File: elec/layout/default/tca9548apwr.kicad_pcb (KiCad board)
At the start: 2 copper layers, 20 parts

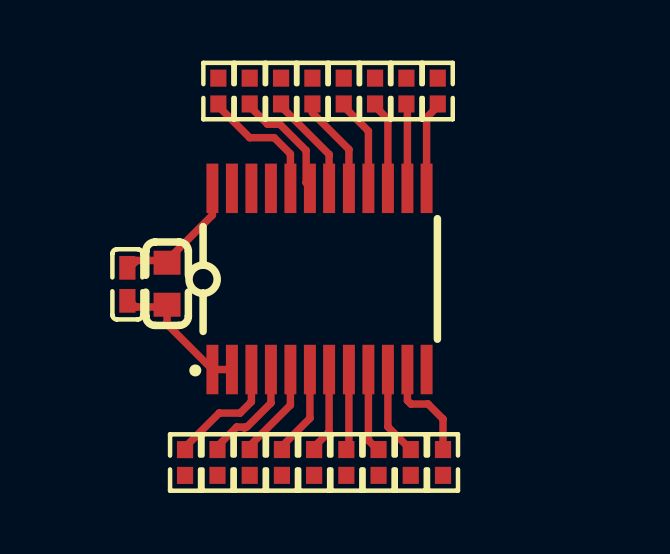
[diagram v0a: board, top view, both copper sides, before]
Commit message: Fix frozen
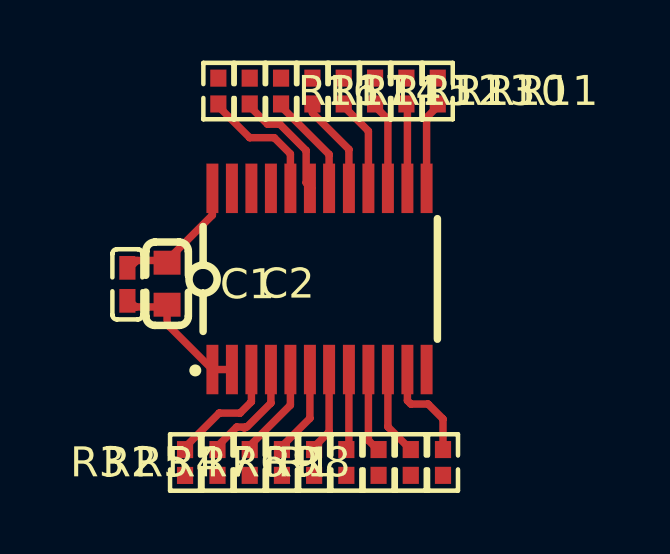
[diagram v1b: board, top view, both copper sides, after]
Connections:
- R1 pad 1: RESET_ -> line-13
- R10 pad 1: hv -> line-10
- R10 pad 2: line-1 -> hv
- R11 pad 1: hv -> line-8
- R11 pad 2: line-13 -> hv
- R12 pad 1: hv -> line
- R12 pad 2: line-5 -> hv
- R13 pad 1: hv -> line-16
- R13 pad 2: line-7 -> hv
- R14 pad 1: hv -> line-2
- R14 pad 2: line-14 -> hv
- R15 pad 1: hv -> line-3
- R15 pad 2: line-10 -> hv
- R16 pad 1: hv -> line-5
- R16 pad 2: line-9 -> hv
- R17 pad 1: hv -> line-15
- R17 pad 2: line-8 -> hv
- R2 pad 1: hv -> line-14
- R2 pad 2: line -> hv
- R3 pad 1: hv -> line-4
- R3 pad 2: line-15 -> hv
- R4 pad 1: hv -> line-12
- R4 pad 2: line-12 -> hv
- R5 pad 1: hv -> line-1
- R5 pad 2: line-4 -> hv
- R6 pad 1: hv -> line-9
- R6 pad 2: line-3 -> hv
- R7 pad 1: hv -> line-7
- R7 pad 2: line-11 -> hv
- R8 pad 1: hv -> line-11
- R8 pad 2: line-6 -> hv
- R9 pad 1: hv -> line-6
- R9 pad 2: line-2 -> hv
- U1 pad 10: line-2 -> line-6
- U1 pad 11: line-6 -> line-11
- U1 pad 13: line-13 -> line-8
- U1 pad 14: line-1 -> line-10
- U1 pad 15: line-7 -> line-16
- U1 pad 16: line-5 -> line
- U1 pad 17: line-10 -> line-3
- U1 pad 18: line-14 -> line-2
- U1 pad 19: line-8 -> line-15
- U1 pad 20: line-9 -> line-5
- U1 pad 3: RESET_ -> line-13
- U1 pad 4: line-15 -> line-4
- U1 pad 5: line -> line-14
- U1 pad 6: line-4 -> line-1
- U1 pad 8: line-11 -> line-7
- U1 pad 9: line-3 -> line-9
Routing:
- net (no net): track 0.00 -> 31.6 mm
- net line-9: track 4.21 -> 0.00 mm
- net line-13: track 2.89 -> 6.80 mm
- net RESET_: track 3.91 -> 0.00 mm
- net line-15: track 3.51 -> 0.00 mm
- net line-6: track 3.42 -> 0.00 mm
- net line-14: track 3.40 -> 0.00 mm
- net line-4: track 2.99 -> 0.00 mm
- net line-2: track 2.94 -> 0.00 mm
- net line-7: track 2.91 -> 0.00 mm
- net line-3: track 2.78 -> 0.00 mm
- net line-1: track 2.75 -> 0.00 mm
- net line-11: track 2.70 -> 0.00 mm
